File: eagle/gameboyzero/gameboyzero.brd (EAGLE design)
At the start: 71 x 94 mm, 27 parts

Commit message: Wed 25 Oct 2017 09:07:01 EDT - holiday express board released
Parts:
- R1: value 1K -> 3R9
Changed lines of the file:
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@@
 </autorouter>
 <elements>
-<element name="R1" library="adafruit" library_urn="urn:adsk.eagle:library:420" package="R0805" value="1K" x="2.6" y="36.5" smashed="yes" rot="R180"/>
+<element name="R1" library="adafruit" library_urn="urn:adsk.eagle:library:420" package="R0805" value="3R9" x="2.6" y="36.5" smashed="yes" rot="R180"/>
 <element name="PI1" library="RPI-Zero" package="RASPBERRYPI_BASTELSTUBE_V13_RASPI_BOARD_B+_FULL" value="RPI-ZERO" x="0.445" y="88.27" rot="MR180"/>
 <element name="SCREEN1" library="GameboyZeroHandheldDisplays" package="GAMEBOYZEROHANDHELDDISPLAYS-2.8" value="GAMEBOYZEROHANDHELDDISPLAYS-2.8" x="35.5" y="63" smashed="yes"/>

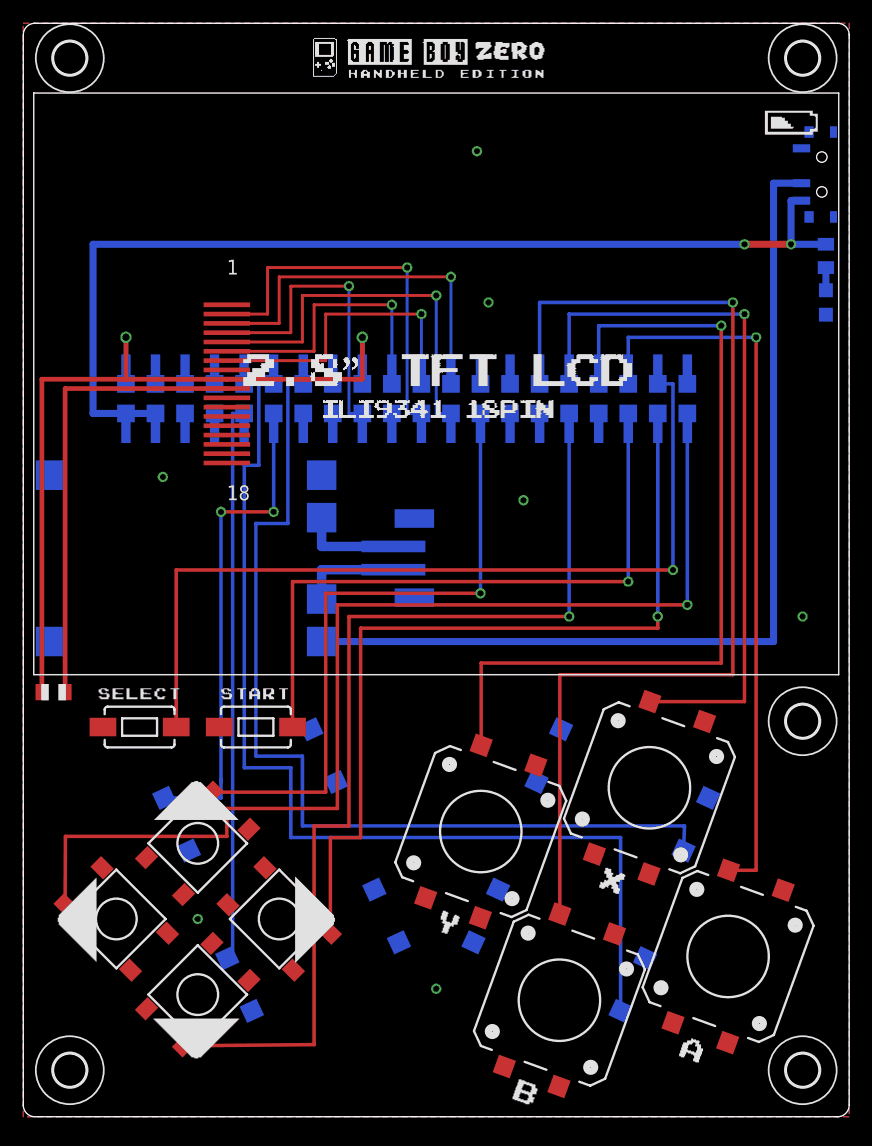
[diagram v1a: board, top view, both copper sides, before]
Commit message: updates
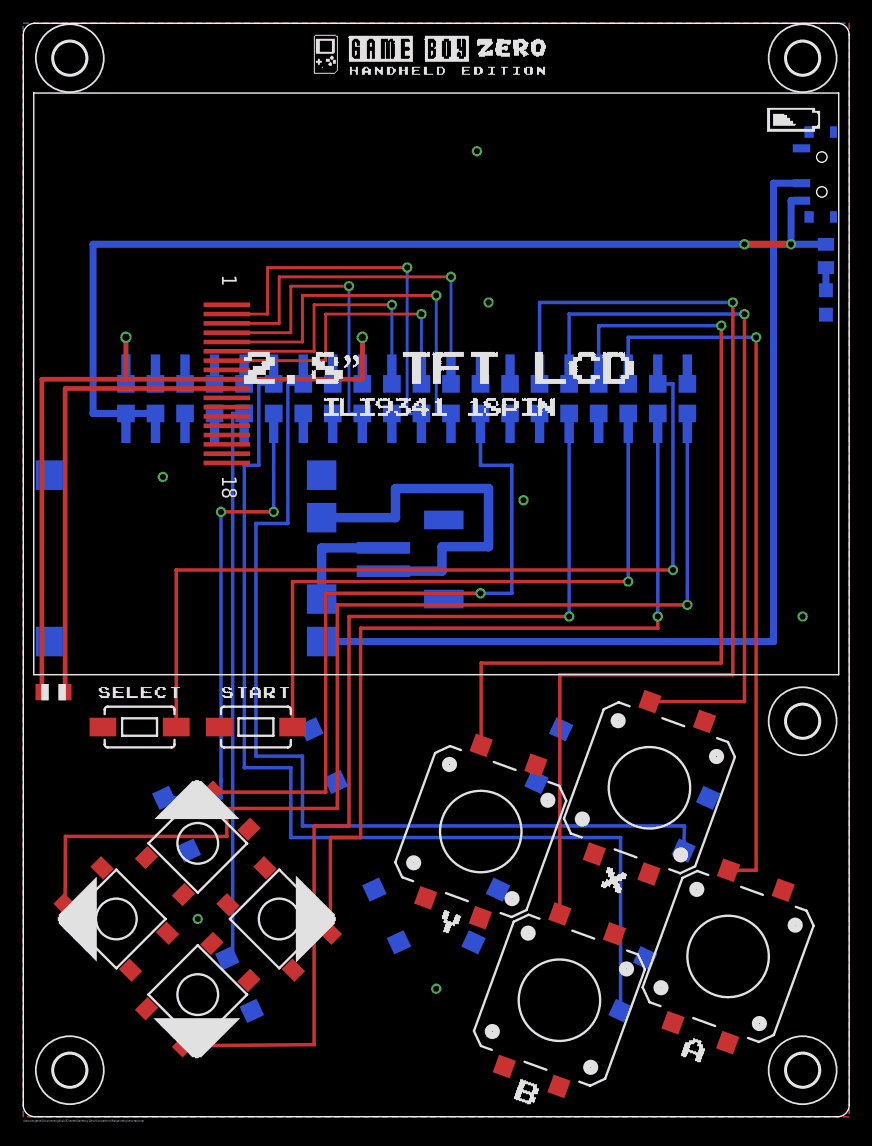
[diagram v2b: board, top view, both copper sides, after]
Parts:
- removed CN1: (no value), adafruit:JST-PH-2-SMT
- added J1: (no value), SparkFun-Connectors:JST-2-SMD
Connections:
- net BATT+: now also J1.2; no longer CN1.1
- net BATT-: now also J1.1; no longer CN1.2
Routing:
- net BATT-: track 8.65 -> 33.0 mm
- net UP: track 55.8 -> 61.0 mm
- net BATT+: track 8.70 -> 9.71 mm
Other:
- board text added: "/Users/eugene/Documents/github/32teeth/Gameboy-Zero-Kickstarter/silks/gameboyzero-bottom.bmp"
- board text added: "/Users/eugene/Documents/github/32teeth/Gameboy-Zero-Kickstarter/silks/gameboyzero-top.bmp"
